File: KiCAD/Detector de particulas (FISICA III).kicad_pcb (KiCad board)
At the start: 2 copper layers, 66 x 21.7 mm, 22 parts, among them J1 Conn_01x02_Female, J2 Conn_01x02_Female, U1 OPA2134PA

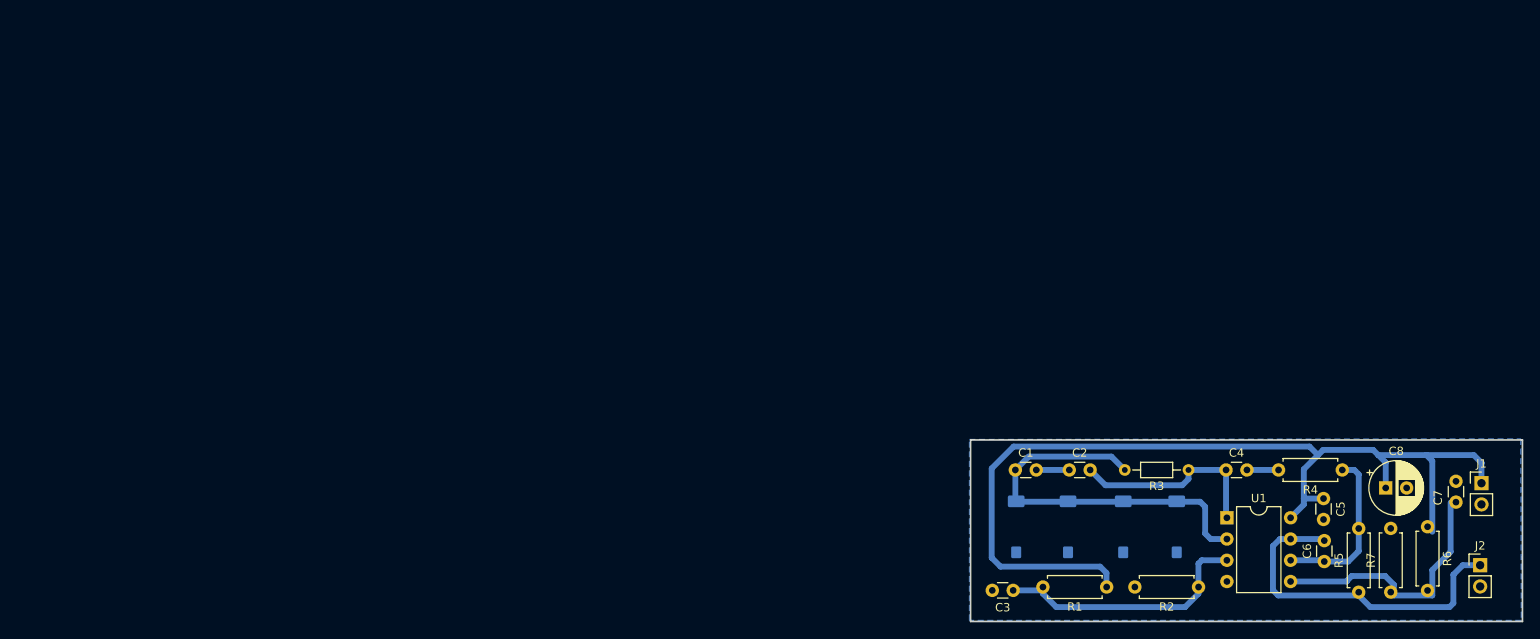
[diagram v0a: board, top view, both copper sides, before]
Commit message: nuevo pcb
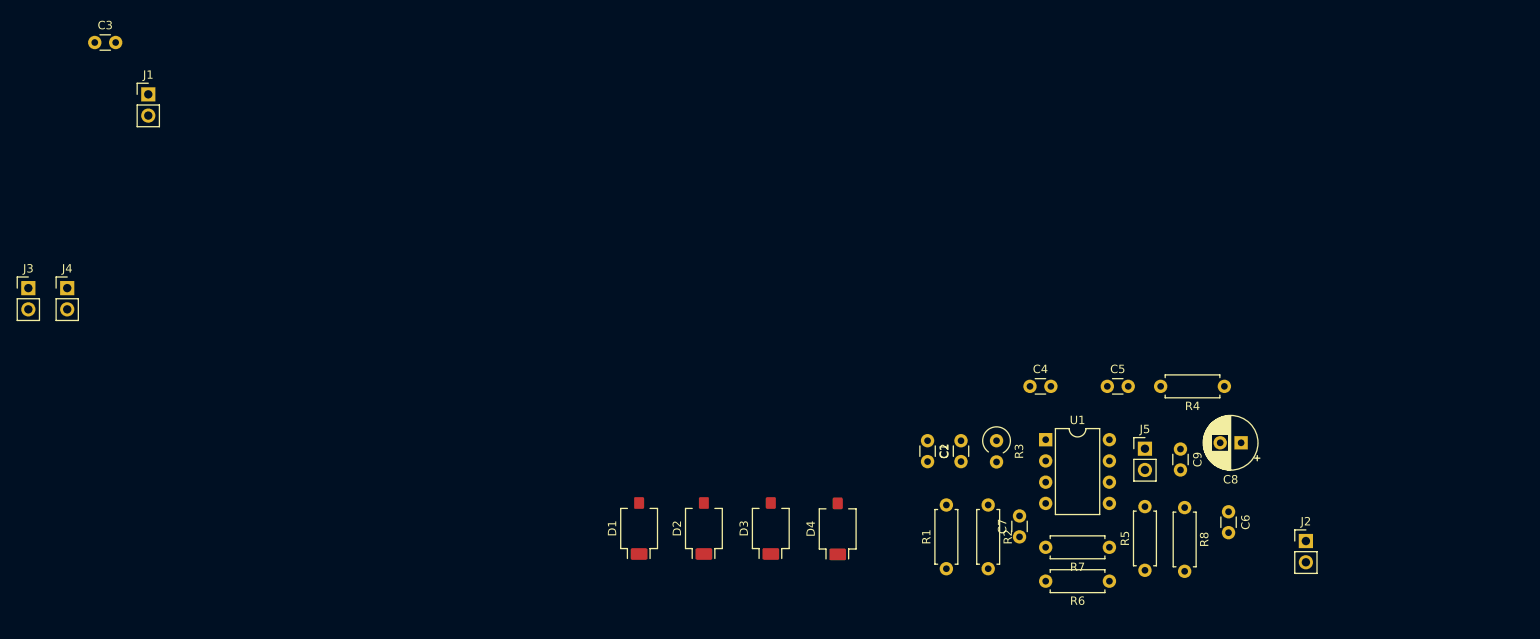
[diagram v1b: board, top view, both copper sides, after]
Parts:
- added C9: 100n, Capacitor_THT:C_Disc_D3.0mm_W1.6mm_P2.50mm, F.Cu at (150.8, 56.0)
- added J3: Conn_01x02_Pin, Connector_PinHeader_2.54mm:PinHeader_1x02_P2.54mm_Vertical, F.Cu at (12.9, 36.8)
- added J4: Conn_01x02_Pin, Connector_PinHeader_2.54mm:PinHeader_1x02_P2.54mm_Vertical, F.Cu at (17.6, 36.8)
- added J5: Conn_01x02_Pin, Connector_PinHeader_2.54mm:PinHeader_1x02_P2.54mm_Vertical, F.Cu at (146.5, 56.0)
- added R8: 2k2, Resistor_THT:R_Axial_DIN0207_L6.3mm_D2.5mm_P7.62mm_Horizontal, F.Cu at (151.2, 63.0)
- D1, D2, D3, D4: moved to F.Cu
- R3: footprint Resistor_THT:R_Axial_DIN0204_L3.6mm_D1.6mm_P7.62mm_Horizontal -> Resistor_THT:R_Axial_DIN0309_L9.0mm_D3.2mm_P2.54mm_Vertical
- moved J1 166.1 mm to (27.3, 13.6)
- moved C3 127.9 mm to (20.9, 7.38), turned to 0 degrees
- moved D1 64.3 mm to (86.0, 65.5), turned to 90 degrees
- moved C7 52.4 mm to (131.5, 66.5)
- moved D2 50.2 mm to (93.8, 65.5), turned to 90 degrees
- moved R6 38.6 mm to (142.2, 71.8), turned to 180 degrees
- moved D3 35.6 mm to (101.8, 65.5), turned to 90 degrees
- moved R7 34.1 mm to (142.2, 67.8), turned to 180 degrees
- moved C5 29.1 mm to (142.0, 48.5), turned to 0 degrees
- moved R2 27.0 mm to (127.8, 62.7), turned to -90 degrees
- moved R5 25.7 mm to (146.5, 70.5)
- moved C4 25.5 mm to (132.8, 48.5)
- moved U1 23.6 mm to (134.6, 54.9)
- moved R3 23.2 mm to (128.8, 55.0), turned to -90 degrees
- moved D4 21.4 mm to (109.8, 65.5), turned to 90 degrees
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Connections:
- C1 pad 1: Net-(D1-K) -> Net-(J3-Pin_1)
- C6 pad 2: /Output -> Net-(J5-Pin_2)
- J1 pad 1: +9V -> Net-(J1-Pin_1)
- R3 pad 2: Net-(D1-K) -> Net-(J3-Pin_1)
- R5 pad 1: /Output -> Net-(J5-Pin_2)
- U1 pad 2: Net-(D1-K) -> Net-(J3-Pin_1)
- U1 pad 7: /Output -> Net-(J5-Pin_2)
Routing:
- net +9V: track 114.7 -> 0.00 mm
- net Net-(D1-K): track 47.7 -> 0.00 mm
- net /Output: track 41.5 -> 0.00 mm
- net Net-(U1-In1+): track 31.0 -> 0.00 mm
- net Net-(U1-In2+): track 31.0 -> 0.00 mm
- net Net-(U1-Out1): track 24.6 -> 0.00 mm
- net Net-(U1-In2-): track 20.1 -> 0.00 mm
- net Net-(C1-Pad2): track 3.95 -> 0.00 mm
- net Net-(C4-Pad2): track 3.78 -> 0.00 mm
- removed copper zone on B.Cu, net GND
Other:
- board outline removed
